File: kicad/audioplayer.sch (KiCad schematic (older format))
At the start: 24 parts, among them J1 Panel, J2 Charge_USB, J3 Speakers, SW1 POWER, U1 PB-500, U2 ESP32-nodeMCU, U3 OLED, U4 GY-521, U5 VS1053/SD_breakout, U6 RC-552_breakout, U7 HW-323

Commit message: first board revision completed
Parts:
- removed U6: RC-552_breakout, symbol audioplayer:RC-552
- added C3, C4, C5, C6, C7: C, Capacitor_THT:C_Disc_D5.1mm_W3.2mm_P5.00mm, symbol Device:C
- added C8: 1u, Capacitor_THT:C_Rect_L7.2mm_W5.5mm_P5.00mm_FKS2_FKP2_MKS2_MKP2, symbol Device:C
- added J4: RFID, Connector_PinHeader_2.54mm:PinHeader_2x05_P2.54mm_Vertical, symbol Connector_Generic:Conn_02x05_Odd_Even
- C1: renamed from 100u1; value CP -> 100u; footprint (none) -> Capacitor_THT:CP_Radial_D10.0mm_P5.00mm
- C2: renamed from 470u1; value CP -> 470u; footprint (none) -> Capacitor_THT:CP_Radial_D10.0mm_P5.00mm
- J1: footprint (none) -> Connector_PinHeader_2.54mm:PinHeader_2x05_P2.54mm_Vertical
- J2, SW1: footprint (none) -> Connector_PinHeader_2.54mm:PinHeader_1x02_P2.54mm_Vertical
- J3, U3: footprint (none) -> Connector_PinHeader_2.54mm:PinHeader_1x04_P2.54mm_Vertical
- L1, L2: footprint (none) -> Inductor_THT:L_Axial_L6.6mm_D2.7mm_P10.16mm_Horizontal_Vishay_IM-2
- R1: value 100k -> 10k; footprint (none) -> Resistor_THT:R_Axial_DIN0204_L3.6mm_D1.6mm_P5.08mm_Horizontal
- R2: value 330k -> 33k; footprint (none) -> Resistor_THT:R_Axial_DIN0204_L3.6mm_D1.6mm_P5.08mm_Horizontal
- R3, R4, R5, R6, R7, R8, R9: footprint (none) -> Resistor_THT:R_Axial_DIN0204_L3.6mm_D1.6mm_P5.08mm_Horizontal
- U1: footprint (none) -> audioplayer:adafruit-pb500-charge
- U2: footprint (none) -> audioplayer:esp32-nodemcu
- U4: footprint (none) -> audioplayer:gy-521
- U5: footprint (none) -> audioplayer:vs1053_breakout_upside_down
- U7: footprint (none) -> audioplayer:hw-323
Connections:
- net labels added: MP3_DREQ, MP3_XCS, MP3_XDCS, MP3_XRESET, RST, SD_CS, SS, VCC_AMP, VCC_MP3
- wire segments 136 -> 171
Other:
- moved on the sheet: C1, L1, L2, R1, R2, R3, R4, R5, R6, R7, R8, U4

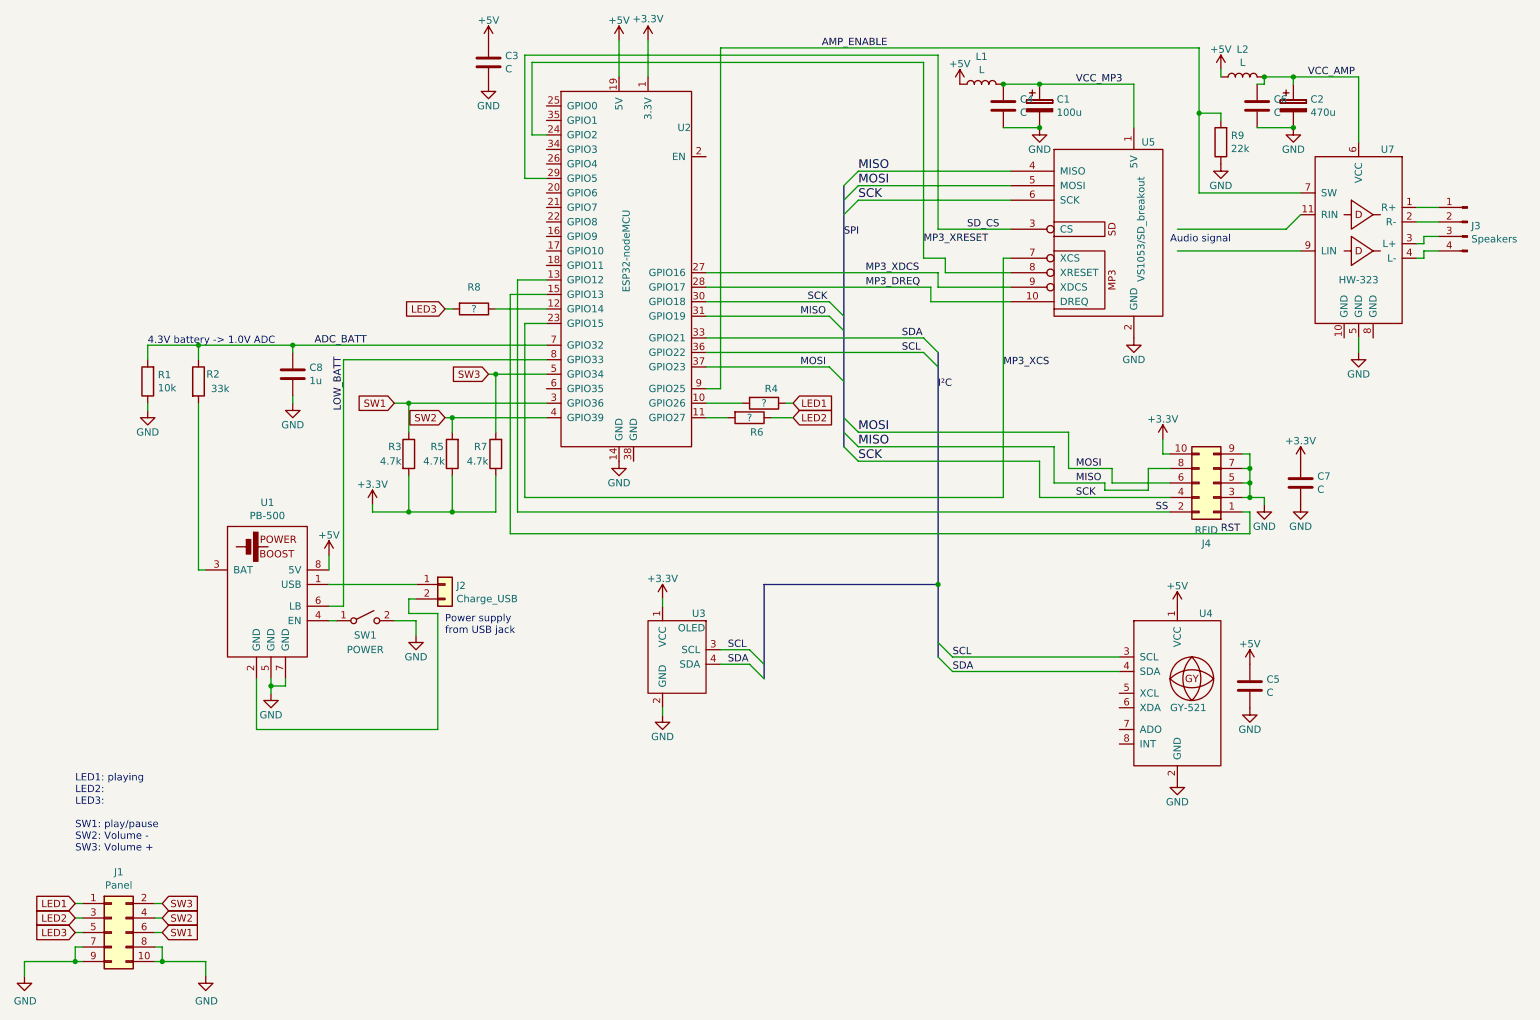
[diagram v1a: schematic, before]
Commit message: board improvements
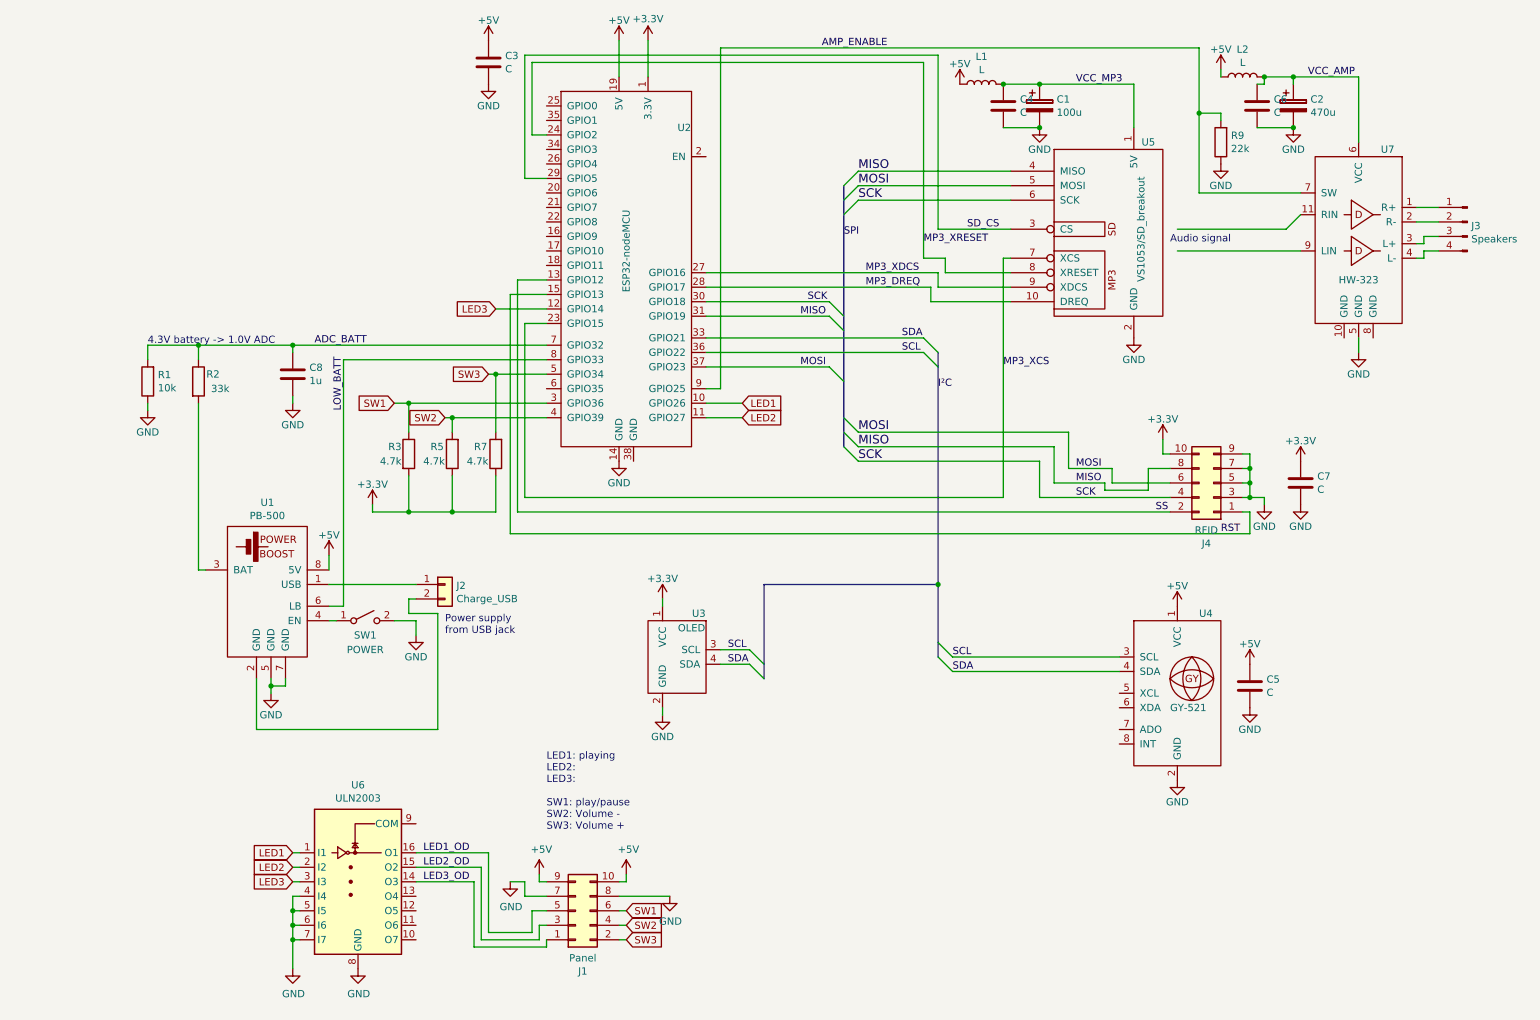
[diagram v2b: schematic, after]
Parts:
- removed R4, R6, R8: ?, Resistor_THT:R_Axial_DIN0204_L3.6mm_D1.6mm_P5.08mm_Horizontal, symbol Device:R
- added U6: ULN2003, Package_DIP:DIP-16_W7.62mm, symbol Transistor_Array:ULN2003
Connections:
- net +5V: now also J1.10 (Pin_10), J1.9 (Pin_9)
- net GND: now also U6.4 (I4), U6.5 (I5), U6.6 (I6), U6.7 (I7), U6.8 (GND); no longer J1.10 (Pin_10), J1.9 (Pin_9)
- net LED1: now also U2.10 (GPIO26), U6.1 (I1); no longer J1.1 (Pin_1)
- net LED2: now also U2.11 (GPIO27), U6.2 (I2); no longer J1.3 (Pin_3)
- net LED3: now also U2.12 (GPIO14), U6.3 (I3); no longer J1.5 (Pin_5)
- new net LED1_OD: J1.5 (Pin_5), U6.16 (O1)
- new net LED2_OD: J1.3 (Pin_3), U6.15 (O2)
- new net LED3_OD: J1.1 (Pin_1), U6.14 (O3)
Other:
- moved on the sheet: J1
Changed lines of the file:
@@
 	1    0    0    -1
-$EndComp
-$Comp
-L Device:R R4
-U 1 1 5BC4BCB4
-P 5850 3250
-F 0 "R4" V 5750 3300 50  0000 C CNN
-F 1 "?" V 5850 3250 50  0000 C CNN
-F 2 "Resistor_THT:R_Axial_DIN0204_L3.6mm_D1.6mm_P5.08mm_Horizontal" V 5780 3250 50  0001 C CNN
-F 3 "" H 5850 3250 50  0001 C CNN
-	1    5850 3250
-	0    1    1    0
-$EndComp
-$Comp
-L Device:R R6
-U 1 1 5BC4BD31
-P 5750 3350
-F 0 "R6" V 5850 3400 50  0000 C CNN
-F 1 "?" V 5750 3350 50  0000 C CNN
-F 2 "Resistor_THT:R_Axial_DIN0204_L3.6mm_D1.6mm_P5.08mm_Horizontal" V 5680 3350 50  0001 C CNN
-F 3 "" H 5750 3350 50  0001 C CNN
-	1    5750 3350
-	0    1    1    0
-$EndComp
-$Comp
-L Device:R R8
-U 1 1 5BC4BD63
-P 3850 2600
-F 0 "R8" V 3700 2600 50  0000 C CNN
-F 1 "?" V 3850 2600 50  0000 C CNN
-F 2 "Resistor_THT:R_Axial_DIN0204_L3.6mm_D1.6mm_P5.08mm_Horizontal" V 3780 2600 50  0001 C CNN
-F 3 "" H 3850 2600 50  0001 C CNN
-	1    3850 2600
-	0    1    1    0
 $EndComp
 Entry Wire Line
@@
 	1    0    0    -1
 $EndComp
-Text GLabel 6050 3250 2    50   Input ~ 0
+Text GLabel 5700 3250 2    50   Input ~ 0
 LED1
-Text GLabel 6050 3350 2    50   Input ~ 0
+Text GLabel 5700 3350 2    50   Input ~ 0
 LED2
-Text GLabel 3650 2600 0    50   Input ~ 0
+Text GLabel 4000 2600 0    50   Input ~ 0
 LED3
 Text GLabel 3300 3250 0    50   Input ~ 0
@@
 Wire Wire Line
 	10400 2200 10500 2200
-$Comp
-L Connector_Generic:Conn_02x05_Odd_Even J1
-U 1 1 5BE80741
-P 1350 6900
-F 0 "J1" H 1400 7317 50  0000 C CNN
-F 1 "Panel" H 1400 7226 50  0000 C CNN
-F 2 "Connector_PinHeader_2.54mm:PinHeader_2x05_P2.54mm_Vertical" H 1350 6900 50  0001 C CNN
-F 3 "~" H 1350 6900 50  0001 C CNN
-	1    1350 6900
-	1    0    0    -1
-$EndComp
-Text GLabel 1100 6700 0    50   Input ~ 0
+Text GLabel 2600 6350 0    50   Input ~ 0
 LED1
-Text GLabel 1100 6800 0    50   Input ~ 0
+Text GLabel 2600 6450 0    50   Input ~ 0
 LED2
-Text GLabel 1700 6900 2    50   Input ~ 0
+Text GLabel 4900 6750 2    50   Input ~ 0
 SW1
-Text GLabel 1100 6900 0    50   Input ~ 0
+Text GLabel 2600 6550 0    50   Input ~ 0
 LED3
-Text GLabel 1700 6800 2    50   Input ~ 0
+Text GLabel 4900 6850 2    50   Input ~ 0
 SW2
-Text GLabel 1700 6700 2    50   Input ~ 0
+Text GLabel 4900 6950 2    50   Input ~ 0
 SW3
 $Comp
 L power:GND #PWR03
 U 1 1 5BE91661
-P 2000 7200
-F 0 "#PWR03" H 2000 6950 50  0001 C CNN
-F 1 "GND" H 2005 7027 50  0000 C CNN
-F 2 "" H 2000 7200 50  0001 C CNN
-F 3 "" H 2000 7200 50  0001 C CNN
-	1    2000 7200
-	1    0    0    -1
-$EndComp
-$Comp
-L power:GND #PWR01
-U 1 1 5BE91694
-P 750 7200
-F 0 "#PWR01" H 750 6950 50  0001 C CNN
-F 1 "GND" H 755 7027 50  0000 C CNN
-F 2 "" H 750 7200 50  0001 C CNN
-F 3 "" H 750 7200 50  0001 C CNN
-	1    750  7200
-	1    0    0    -1
-$EndComp
-Text Notes 1100 6350 0    50   ~ 0
+P 5200 6650
+F 0 "#PWR03" H 5200 6400 50  0001 C CNN
+F 1 "GND" H 5205 6477 50  0000 C CNN
+F 2 "" H 5200 6650 50  0001 C CNN
+F 3 "" H 5200 6650 50  0001 C CNN
+	1    5200 6650
+	1    0    0    -1
+$EndComp
+Text Notes 4350 6200 0    50   ~ 0
 LED1: playing\nLED2: \nLED3: \n\nSW1: play/pause\nSW2: Volume -\nSW3: Volume +
 Wire Wire Line
@@
 Wire Wire Line
 	3300 3250 3400 3250
-$Comp
-L power:+3.3V #PWR07
-U 1 1 5C0A7548
-P 3150 3950
-F 0 "#PWR07" H 3150 3800 50  0001 C CNN
-F 1 "+3.3V" H 3150 4090 50  0000 C CNN
-F 2 "" H 3150 3950 50  0000 C CNN
-F 3 "" H 3150 3950 50  0000 C CNN
-	1    3150 3950
-	1    0    0    -1
-$EndComp
 $Comp
 L Device:R R3
@@
 	6300 2650 5450 2650
 Wire Wire Line
-	5450 3250 5700 3250
-Wire Wire Line
-	5900 3350 6050 3350
-Wire Wire Line
-	6050 3250 6000 3250
-Wire Wire Line
 	7150 5100 8300 5100
 Wire Wire Line
@@
 	4000 2600 4350 2600
 Wire Wire Line
-	3650 2600 3700 2600
-Wire Wire Line
 	3150 3950 3150 4000
 Wire Wire Line
@@
 Wire Wire Line
 	4000 3450 4000 3050
-Wire Wire Line
-	5450 3350 5600 3350
 $Comp
 L Connector_Generic:Conn_02x05_Odd_Even J4
@@
 Wire Wire Line
 	2350 5150 2350 5500
-Wire Wire Line
-	1650 6700 1700 6700
-Wire Wire Line
-	1650 6800 1700 6800
-Wire Wire Line
-	1650 6900 1700 6900
-Wire Wire Line
-	1100 6700 1150 6700
-Wire Wire Line
-	1150 6800 1100 6800
-Wire Wire Line
-	1100 6900 1150 6900
-Wire Wire Line
-	2000 7200 2000 7100
-Wire Wire Line
-	2000 7100 1700 7100
-Wire Wire Line
-	1650 7000 1700 7000
-Wire Wire Line
-	1700 7000 1700 7100
-Connection ~ 1700 7100
-Wire Wire Line
-	1700 7100 1650 7100
-Wire Wire Line
-	750  7200 750  7100
-Wire Wire Line
-	750  7100 1100 7100
-Wire Wire Line
-	1150 7000 1100 7000
-Wire Wire Line
-	1100 7000 1100 7100
-Connection ~ 1100 7100
-Wire Wire Line
-	1100 7100 1150 7100
 Text Label 7250 2050 0    50   ~ 0
 SD_CS
@@
 Wire Wire Line
 	2600 3250 2600 3200
+$Comp
+L Transistor_Array:ULN2003 U6
+U 1 1 5BEE63E1
+P 3050 6550
+F 0 "U6" H 3050 7217 50  0000 C CNN
+F 1 "ULN2003" H 3050 7126 50  0000 C CNN
+F 2 "Package_DIP:DIP-16_W7.62mm" H 3100 6000 50  0001 L CNN
+F 3 "http://www.ti.com/lit/ds/symlink/uln2003a.pdf" H 3150 6350 50  0001 C CNN
+	1    3050 6550
+	1    0    0    -1
+$EndComp
+Wire Wire Line
+	2600 6350 2650 6350
+Wire Wire Line
+	2600 6450 2650 6450
+Wire Wire Line
+	2600 6550 2650 6550
+$Comp
+L power:GND #PWR0110
+U 1 1 5BF348CC
+P 3050 7150
+F 0 "#PWR0110" H 3050 6900 50  0001 C CNN
+F 1 "GND" H 3055 6977 50  0000 C CNN
+F 2 "" H 3050 7150 50  0001 C CNN
+F 3 "" H 3050 7150 50  0001 C CNN
+	1    3050 7150
+	1    0    0    -1
+$EndComp
+Wire Wire Line
+	5450 3350 5700 3350
+Wire Wire Line
+	5450 3250 5700 3250
+$Comp
+L Connector_Generic:Conn_02x05_Odd_Even J1
+U 1 1 5BE80741
+P 4550 6750
+F 0 "J1" H 4600 7167 50  0000 C CNN
+F 1 "Panel" H 4600 7076 50  0000 C CNN
+F 2 "Connector_PinHeader_2.54mm:PinHeader_2x05_P2.54mm_Vertical" H 4550 6750 50  0001 C CNN
+F 3 "~" H 4550 6750 50  0001 C CNN
+	1    4550 6750
+	1    0    0    1
+$EndComp
+Text Label 3500 6350 0    50   ~ 0
+LED1_OD
+Text Label 3500 6450 0    50   ~ 0
+LED2_OD
+Text Label 3500 6550 0    50   ~ 0
+LED3_OD
+$Comp
+L power:GND #PWR0112
+U 1 1 5C0819A7
+P 4100 6550
+F 0 "#PWR0112" H 4100 6300 50  0001 C CNN
+F 1 "GND" H 4105 6377 50  0000 C CNN
+F 2 "" H 4100 6550 50  0001 C CNN
+F 3 "" H 4100 6550 50  0001 C CNN
+	1    4100 6550
+	1    0    0    -1
+$EndComp
+Wire Wire Line
+	3450 6550 3850 6550
+Wire Wire Line
+	3450 6450 3900 6450
+Wire Wire Line
+	3450 6350 3950 6350
+$Comp
+L power:+5V #PWR0109
+U 1 1 5C1F71E9
+P 4300 6500
+F 0 "#PWR0109" H 4300 6350 50  0001 C CNN
+F 1 "+5V" H 4315 6673 50  0000 C CNN
+F 2 "" H 4300 6500 50  0001 C CNN
+F 3 "" H 4300 6500 50  0001 C CNN
+	1    4300 6500
+	1    0    0    -1
+$EndComp
+$Comp
+L power:+5V #PWR0111
+U 1 1 5C1FFDF2
+P 4900 6500
+F 0 "#PWR0111" H 4900 6350 50  0001 C CNN
+F 1 "+5V" H 4915 6673 50  0000 C CNN
+F 2 "" H 4900 6500 50  0001 C CNN
+F 3 "" H 4900 6500 50  0001 C CNN
+	1    4900 6500
+	1    0    0    -1
+$EndComp
+$Comp
+L power:+3.3V #PWR07
+U 1 1 5C0A7548
+P 3150 3950
+F 0 "#PWR07" H 3150 3800 50  0001 C CNN
+F 1 "+3.3V" H 3150 4090 50  0000 C CNN
+F 2 "" H 3150 3950 50  0000 C CNN
+F 3 "" H 3150 3950 50  0000 C CNN
+	1    3150 3950
+	1    0    0    -1
+$EndComp
+Wire Wire Line
+	4850 6550 4900 6550
+Wire Wire Line
+	4900 6550 4900 6500
+Wire Wire Line
+	4300 6500 4300 6550
+Wire Wire Line
+	4300 6550 4350 6550
+Wire Wire Line
+	4850 6650 5200 6650
+Wire Wire Line
+	3950 6900 4250 6900
+Wire Wire Line
+	4250 6900 4250 6750
+Wire Wire Line
+	4250 6750 4350 6750
+Wire Wire Line
+	3950 6350 3950 6900
+Wire Wire Line
+	3900 6450 3900 6950
+Wire Wire Line
+	3900 6950 4300 6950
+Wire Wire Line
+	4300 6950 4300 6850
+Wire Wire Line
+	4300 6850 4350 6850
+Wire Wire Line
+	4350 6950 4350 7000
+Wire Wire Line
+	4350 7000 3850 7000
+Wire Wire Line
+	3850 6550 3850 7000
+Wire Wire Line
+	4100 6550 4200 6550
+Wire Wire Line
+	4200 6550 4200 6650
+Wire Wire Line
+	4200 6650 4350 6650
+Wire Wire Line
+	4850 6750 4900 6750
+Wire Wire Line
+	4900 6850 4850 6850
+Wire Wire Line
+	4850 6950 4900 6950
+Wire Wire Line
+	2650 6650 2600 6650
+Wire Wire Line
+	2600 6650 2600 6750
+Wire Wire Line
+	2650 6950 2600 6950
+Connection ~ 2600 6950
+Wire Wire Line
+	2600 6950 2600 7150
+Wire Wire Line
+	2650 6850 2600 6850
+Connection ~ 2600 6850
+Wire Wire Line
+	2600 6850 2600 6950
+Wire Wire Line
+	2650 6750 2600 6750
 Wire Bus Line
 	7050 2900 7050 4500
@@
 Wire Bus Line
 	6400 1750 6400 3550
+Connection ~ 2600 6750
+Wire Wire Line
+	2600 6750 2600 6850
+$Comp
+L power:GND #PWR?
+U 1 1 5C5B1938
+P 2600 7150
+F 0 "#PWR?" H 2600 6900 50  0001 C CNN
+F 1 "GND" H 2605 6977 50  0000 C CNN
+F 2 "" H 2600 7150 50  0001 C CNN
+F 3 "" H 2600 7150 50  0001 C CNN
+	1    2600 7150
+	1    0    0    -1
+$EndComp
 $EndSCHEMATC
